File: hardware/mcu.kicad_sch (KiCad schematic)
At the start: 24 parts, among them J2001 USB_C_Receptacle_USB2.0_14P, J2002 CAN, Q2001 MMBT3904, Q2002 MMBT3904, SW2001 SW_Push, U2001 ESP32-C3, U2002 MCP2562-E-SN

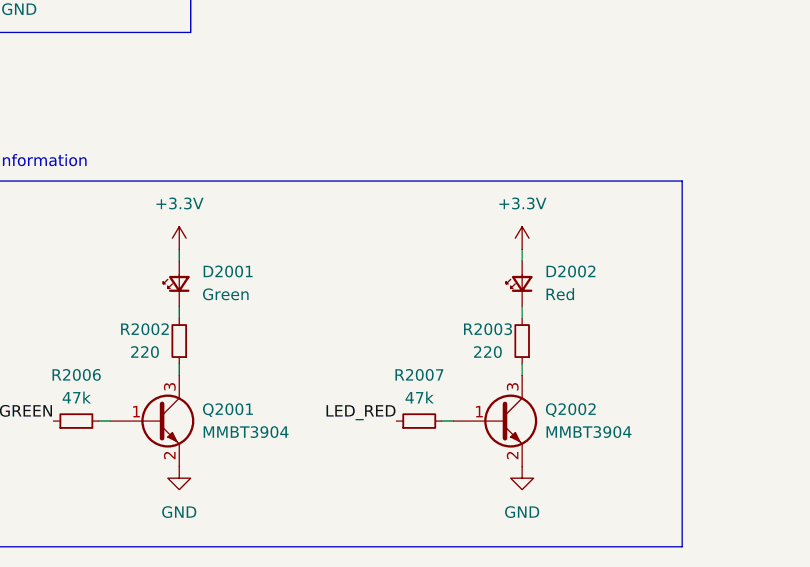
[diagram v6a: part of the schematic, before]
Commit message: Added LDO
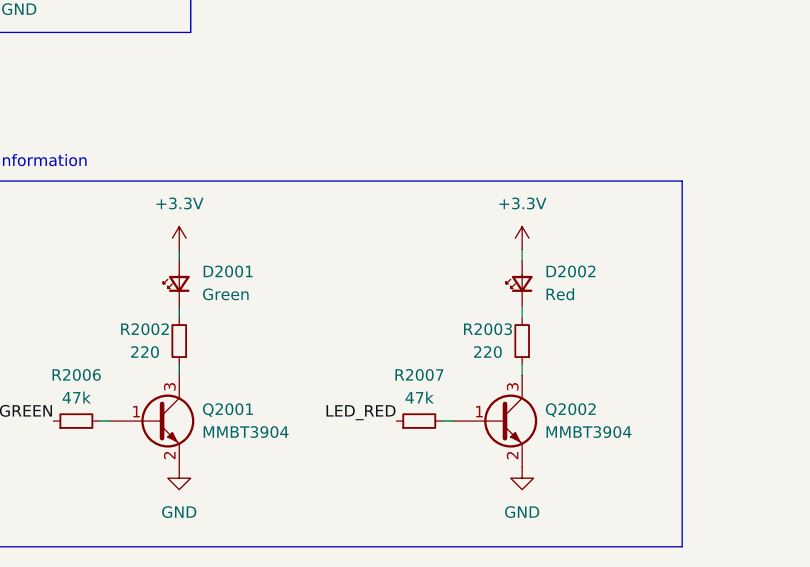
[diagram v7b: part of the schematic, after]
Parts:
- D2001, D2002: footprint LED_THT:LED_D5.0mm -> LED_SMD:LED_0805_2012Metric
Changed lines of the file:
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@@
 	(label "DP"
 		(at 54.61 91.44 180)
+		(fields_autoplaced yes)
 		(effects
 			(font
@@
 	(label "DN"
 		(at 54.61 88.9 180)
+		(fields_autoplaced yes)
 		(effects
 			(font
@@
 		(fields_autoplaced yes)
 		(property "Reference" "D2002"
-			(at 212.09 130.7465 90)
+			(at 212.09 130.7464 90)
 			(effects
 				(font
@@
 		)
 		(property "Value" "Red"
-			(at 212.09 133.2865 90)
+			(at 212.09 133.2864 90)
 			(effects
 				(font
@@
 			)
 		)
-		(property "Footprint" "LED_THT:LED_D5.0mm"
+		(property "Footprint" "LED_SMD:LED_0805_2012Metric"
 			(at 209.55 132.08 90)
 			(effects
@@
 		(fields_autoplaced yes)
 		(property "Reference" "D2001"
-			(at 173.99 130.7465 90)
+			(at 173.99 130.7464 90)
 			(effects
 				(font
@@
 		)
 		(property "Value" "Green"
-			(at 173.99 133.2865 90)
+			(at 173.99 133.2864 90)
 			(effects
 				(font
@@
 			)
 		)
-		(property "Footprint" "LED_THT:LED_D5.0mm"
+		(property "Footprint" "LED_SMD:LED_0805_2012Metric"
 			(at 171.45 132.08 90)
 			(effects
